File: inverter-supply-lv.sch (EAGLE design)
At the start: 62 parts, among them IC3 1039-2387**3.3V 300mA LDO Vol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, U1 1039-2397** MP2456GJ-Z 0.5A, 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, U2 1039-9015**AOZ1282CI Buck Swi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, X1 0289-9066**15EDGVC-3.81-02P-14

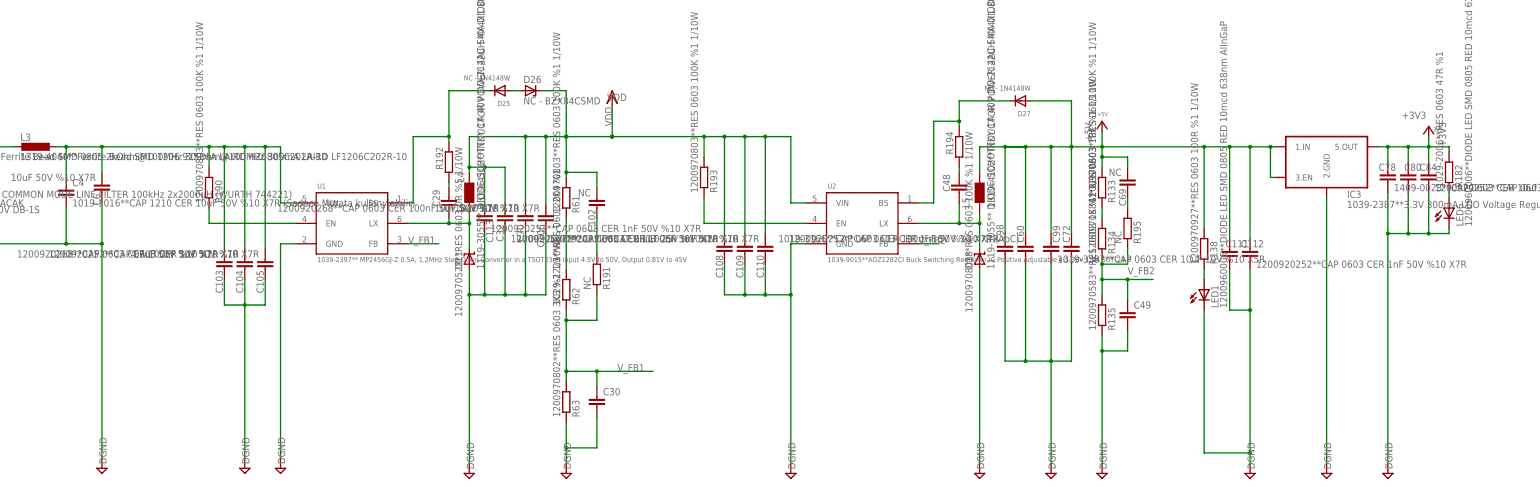
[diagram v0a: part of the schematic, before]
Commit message: Bitti
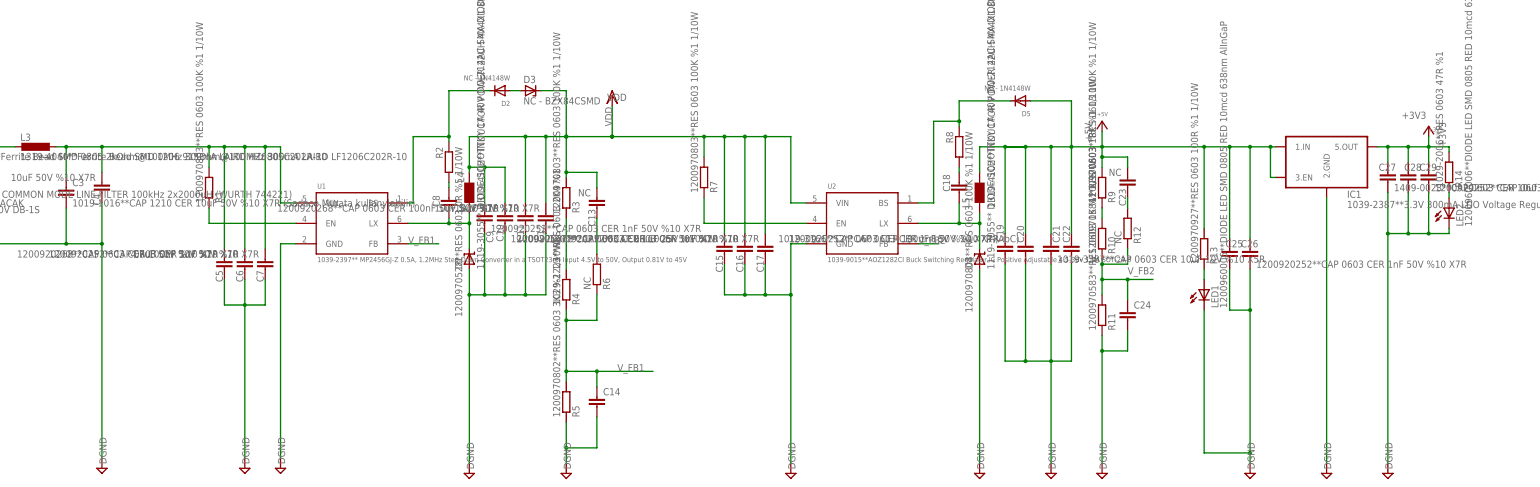
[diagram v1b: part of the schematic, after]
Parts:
- removed C104: 1200920268**CAP 0603 CER 100nF 50V %10 X7R, rcl:C-EUC0603E
- removed C84: 1200920252**CAP 0603 CER 1nF 50V %10 X7R, rcl:C-EUC0603E
- added C3: 1019-1016**CAP 1210 CER 10uF 50V %10 X7R (Sadece Murata kul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, ercl:C-EUC1210
- added C8: 1200920268**CAP 0603 CER 100nF 50V %10 X7R, rcl:C-EUC0603E
- C29: value 1200920268**CAP 0603 CER 100nF 50V %10 X7R -> 1200920252**CAP 0603 CER 1nF 50V %10 X7R
- C4: value 1019-1016**CAP 1210 CER 10uF 50V %10 X7R (Sadece Murata kullanylabilir) -> 10uF 50V %10 X7R; device ercl:C-EUC1210 -> rcl:C-EUC0805E
- C6: value 10uF 50V %10 X7R -> 1200920268**CAP 0603 CER 100nF 50V %10 X7R; device rcl:C-EUC0805E -> rcl:C-EUC0603E
- renumbered C102 to C13, C103 to C5, C105 to C7, C106 to C12, C108 to C15, C109 to C16, C110 to C17, C111 to C25, C112 to C26, C113 to C9, C30 to C14, C32 to C10, C48 to C18, C49 to C24, C60 to C20, C69 to C23, C70 to C11, C72 to C22, C78 to C27, C80 to C28, C98 to C19, C99 to C21, D11 to D1, D18 to D4, D25 to D2, D26 to D3, D27 to D5, IC3 to IC1, LED6 to LED2, R133 to R9, R134 to R10, R135 to R11, R138 to R13, R182 to R14, R190 to R1, R191 to R6, R192 to R2, R193 to R7, R194 to R8, R195 to R12, R61 to R3, R62 to R4, R63 to R5
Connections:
- net +3V3: now also C29.1; no longer C84.1
- net DGND: now also C29.2, C3.1; no longer C104.1, C84.2
- net N$11: now also C8.2; no longer C29.2
- net N$35: now also C8.1; no longer C29.1
- net N$72: now also C3.2; no longer C104.2
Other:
- moved on the sheet: C29, C4, C6
